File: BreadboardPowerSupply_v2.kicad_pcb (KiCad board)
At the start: 2 copper layers, 30.1 x 52.2 mm, 15 parts, among them J1 Barrel_Jack_Switch, J2 Conn_02x02_Odd_Even, J3 Conn_02x02_Odd_Even, SW1 SW_DPDT_x2, U1 LM7805_TO220

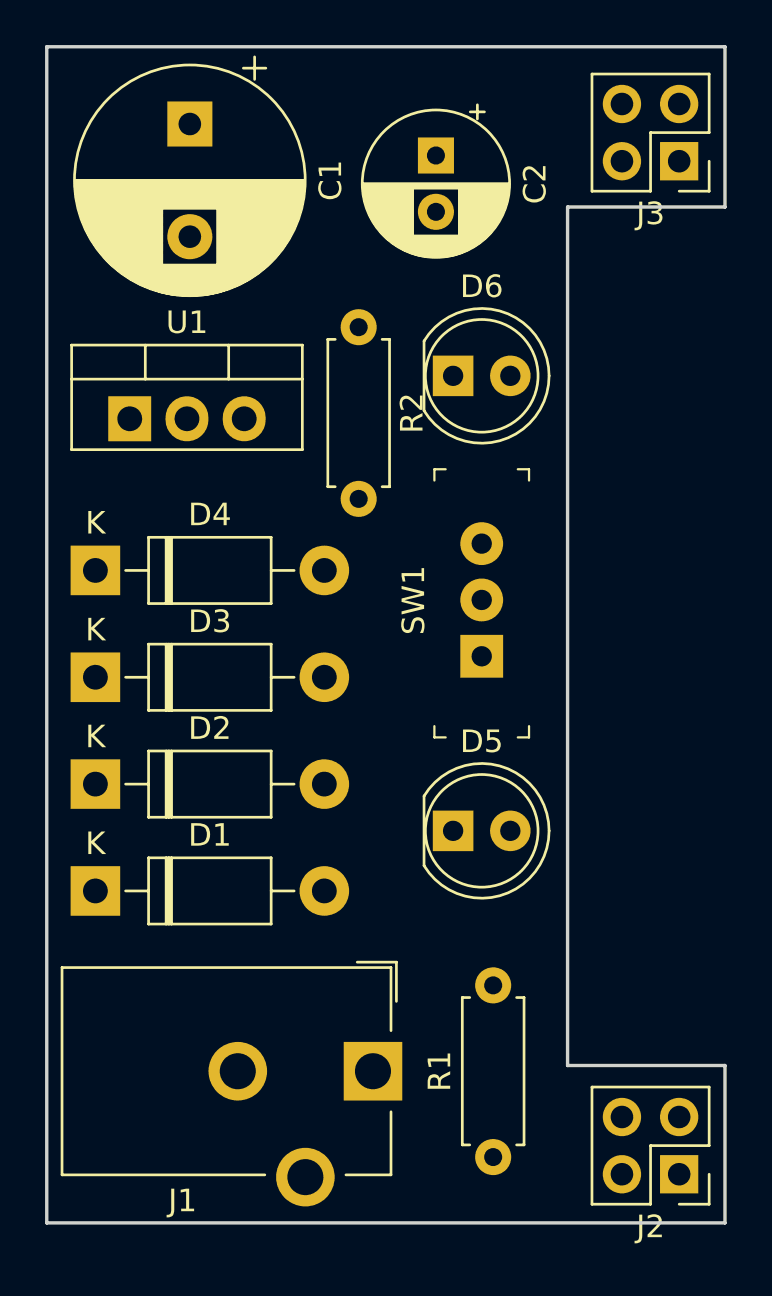
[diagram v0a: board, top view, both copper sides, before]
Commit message: Tracing is complete.
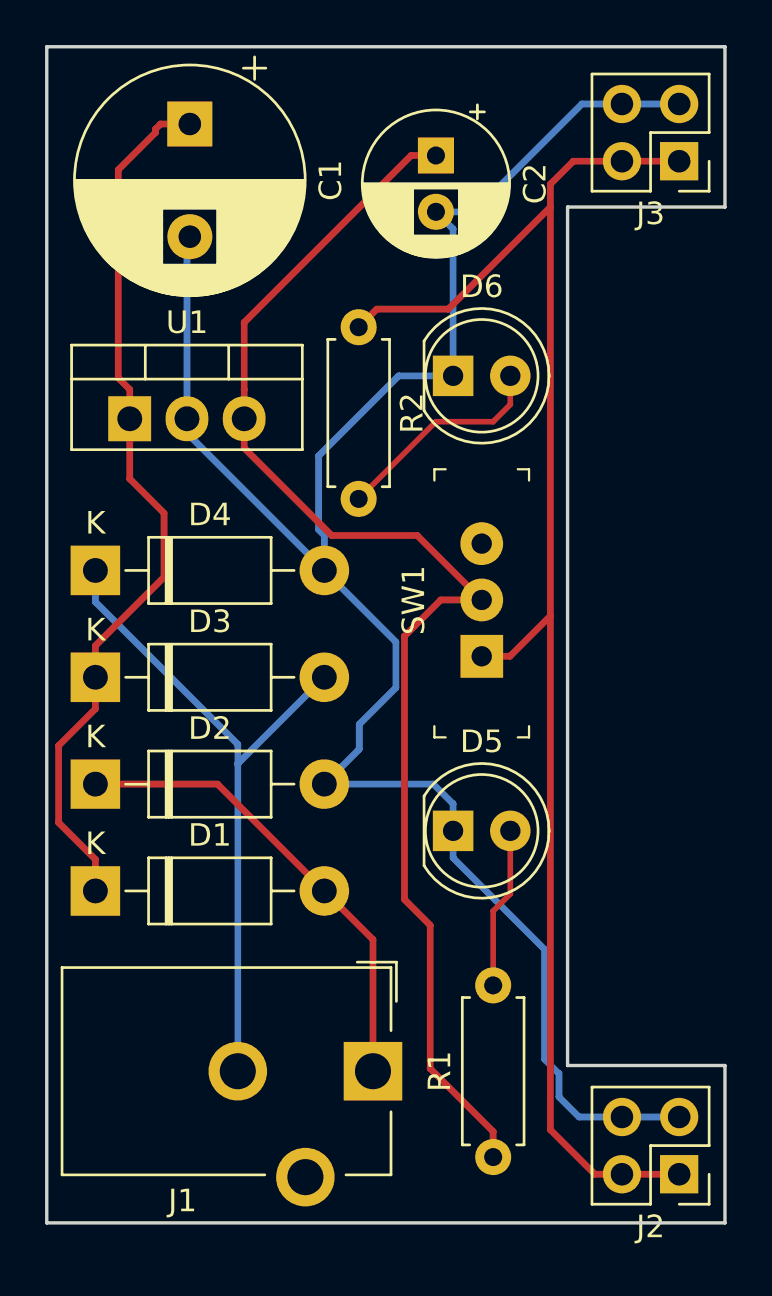
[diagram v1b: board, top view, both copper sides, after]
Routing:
- net /V-: track 0.00 -> 89.2 mm
- net /Vout2: track 0.00 -> 69.1 mm
- net /Vout1: track 0.00 -> 59.3 mm
- net /Vin: track 0.00 -> 39.6 mm
- net /V2: track 0.00 -> 30.3 mm
- net /V1: track 0.00 -> 21.0 mm
- net Net-(D6-Pad2): track 0.00 -> 9.74 mm
- net Net-(D5-Pad2): track 0.00 -> 7.17 mm
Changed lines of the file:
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@@
     (thickness 1.6)
     (drawings 13)
-    (tracks 0)
+    (tracks 93)
     (zones 0)
     (modules 15)
@@
     (uvia_dia 0.3)
     (uvia_drill 0.1)
-    (add_net /V-)
-    (add_net /V1)
-    (add_net /V2)
-    (add_net /Vin)
-    (add_net /Vout1)
-    (add_net /Vout2)
     (add_net "Net-(D5-Pad2)")
     (add_net "Net-(D6-Pad2)")
@@
     (uvia_dia 0.3)
     (uvia_drill 0.1)
+    (add_net /V-)
+    (add_net /V1)
+    (add_net /V2)
+    (add_net /Vin)
+    (add_net /Vout1)
+    (add_net /Vout2)
   )
   (module Capacitor_THT:CP_Radial_D6.3mm_P2.50mm (layer F.Cu)
@@
   (gr_line (start 36.957 159.385) (end 67.056 159.385) (layer Edge.Cuts) (width 0.15))
   (gr_line (start 36.957 107.188) (end 36.957 159.385) (layer Edge.Cuts) (width 0.15))
+  (segment (start 37.48201 141.61901) (end 39.116 143.253) (width 0.3) (layer F.Cu) (net 1))
+  (segment (start 37.48201 138.204323) (end 37.48201 141.61901) (width 0.3) (layer F.Cu) (net 1))
+  (segment (start 39.116 136.570333) (end 37.48201 138.204323) (width 0.3) (layer F.Cu) (net 1))
+  (segment (start 39.116 143.253) (end 39.116 144.653) (width 0.3) (layer F.Cu) (net 1))
+  (segment (start 39.116 135.170333) (end 39.116 136.570333) (width 0.3) (layer F.Cu) (net 1))
+  (segment (start 39.116 133.770333) (end 42.164 130.722333) (width 0.3) (layer F.Cu) (net 1))
+  (segment (start 39.116 135.170333) (end 39.116 133.770333) (width 0.3) (layer F.Cu) (net 1))
+  (segment (start 42.164 130.722333) (end 42.164 127.889) (width 0.3) (layer F.Cu) (net 1))
+  (segment (start 40.64 126.365) (end 40.64 123.698) (width 0.3) (layer F.Cu) (net 1))
+  (segment (start 42.164 127.889) (end 40.64 126.365) (width 0.3) (layer F.Cu) (net 1))
+  (segment (start 42.007 110.617) (end 43.307 110.617) (width 0.3) (layer F.Cu) (net 1))
+  (segment (start 40.132 112.649) (end 41.783 110.998) (width 0.3) (layer F.Cu) (net 1))
+  (segment (start 40.64 122.398) (end 40.132 121.89) (width 0.3) (layer F.Cu) (net 1))
+  (segment (start 40.64 123.698) (end 40.64 122.398) (width 0.3) (layer F.Cu) (net 1))
+  (segment (start 40.132 121.89) (end 40.132 112.649) (width 0.3) (layer F.Cu) (net 1))
+  (segment (start 41.783 110.841) (end 42.007 110.617) (width 0.3) (layer F.Cu) (net 1))
+  (segment (start 41.783 110.998) (end 41.783 110.841) (width 0.3) (layer F.Cu) (net 1))
+  (segment (start 43.18 124.333) (end 43.18 123.698) (width 0.3) (layer B.Cu) (net 2))
+  (segment (start 49.276 130.429) (end 43.18 124.333) (width 0.3) (layer B.Cu) (net 2))
+  (segment (start 54.991 140.786) (end 54.991 141.986) (width 0.3) (layer B.Cu) (net 2))
+  (segment (start 54.116666 139.911666) (end 54.991 140.786) (width 0.3) (layer B.Cu) (net 2))
+  (segment (start 49.276 139.911666) (end 54.116666 139.911666) (width 0.3) (layer B.Cu) (net 2))
+  (segment (start 54.991 143.186) (end 59.055 147.25) (width 0.3) (layer B.Cu) (net 2))
+  (segment (start 54.991 141.986) (end 54.991 143.186) (width 0.3) (layer B.Cu) (net 2))
+  (segment (start 59.055 152.126476) (end 59.69 152.761476) (width 0.3) (layer B.Cu) (net 2))
+  (segment (start 59.055 147.25) (end 59.055 152.126476) (width 0.3) (layer B.Cu) (net 2))
+  (segment (start 59.69 152.761476) (end 59.69 153.797) (width 0.3) (layer B.Cu) (net 2))
+  (segment (start 60.579 154.686) (end 62.484 154.686) (width 0.3) (layer B.Cu) (net 2))
+  (segment (start 59.69 153.797) (end 60.579 154.686) (width 0.3) (layer B.Cu) (net 2))
+  (segment (start 62.484 154.686) (end 65.024 154.686) (width 0.3) (layer B.Cu) (net 2))
+  (segment (start 50.826001 138.361665) (end 50.826001 137.260999) (width 0.3) (layer B.Cu) (net 2))
+  (segment (start 49.276 139.911666) (end 50.826001 138.361665) (width 0.3) (layer B.Cu) (net 2))
+  (segment (start 50.826001 137.260999) (end 52.451 135.636) (width 0.3) (layer B.Cu) (net 2))
+  (segment (start 52.451 133.604) (end 49.276 130.429) (width 0.3) (layer B.Cu) (net 2))
+  (segment (start 52.451 135.636) (end 52.451 133.604) (width 0.3) (layer B.Cu) (net 2))
+  (segment (start 49.276 128.873366) (end 49.022 128.619366) (width 0.3) (layer B.Cu) (net 2))
+  (segment (start 49.276 130.429) (end 49.276 128.873366) (width 0.3) (layer B.Cu) (net 2))
+  (segment (start 49.022 128.619366) (end 49.022 125.349) (width 0.3) (layer B.Cu) (net 2))
+  (segment (start 52.578 121.793) (end 54.991 121.793) (width 0.3) (layer B.Cu) (net 2))
+  (segment (start 49.022 125.349) (end 52.578 121.793) (width 0.3) (layer B.Cu) (net 2))
+  (segment (start 54.991 115.276) (end 54.229 114.514) (width 0.3) (layer B.Cu) (net 2))
+  (segment (start 54.991 121.793) (end 54.991 115.276) (width 0.3) (layer B.Cu) (net 2))
+  (segment (start 43.18 115.744) (end 43.307 115.617) (width 0.3) (layer B.Cu) (net 2))
+  (segment (start 43.18 123.698) (end 43.18 115.744) (width 0.3) (layer B.Cu) (net 2))
+  (segment (start 54.229 114.514) (end 55.92 114.514) (width 0.3) (layer B.Cu) (net 2))
+  (segment (start 55.92 114.514) (end 60.706 109.728) (width 0.3) (layer B.Cu) (net 2))
+  (segment (start 60.706 109.728) (end 62.484 109.728) (width 0.3) (layer B.Cu) (net 2))
+  (segment (start 62.484 109.728) (end 65.024 109.728) (width 0.3) (layer B.Cu) (net 2))
+  (segment (start 56.769 148.844) (end 56.769 145.542) (width 0.25) (layer F.Cu) (net 3))
+  (segment (start 57.531 144.78) (end 57.531 141.986) (width 0.25) (layer F.Cu) (net 3))
+  (segment (start 56.769 145.542) (end 57.531 144.78) (width 0.25) (layer F.Cu) (net 3))
+  (segment (start 57.531 123.065792) (end 56.769 123.827792) (width 0.25) (layer F.Cu) (net 4))
+  (segment (start 57.531 121.793) (end 57.531 123.065792) (width 0.25) (layer F.Cu) (net 4))
+  (segment (start 54.226208 123.827792) (end 50.8 127.254) (width 0.25) (layer F.Cu) (net 4))
+  (segment (start 56.769 123.827792) (end 54.226208 123.827792) (width 0.25) (layer F.Cu) (net 4))
+  (segment (start 51.435 146.812) (end 49.276 144.653) (width 0.3) (layer F.Cu) (net 7))
+  (segment (start 51.435 152.654) (end 51.435 146.812) (width 0.3) (layer F.Cu) (net 7))
+  (segment (start 44.534666 139.911666) (end 39.116 139.911666) (width 0.3) (layer F.Cu) (net 7))
+  (segment (start 49.276 144.653) (end 44.534666 139.911666) (width 0.3) (layer F.Cu) (net 7))
+  (segment (start 45.435 139.011333) (end 49.276 135.170333) (width 0.3) (layer B.Cu) (net 8))
+  (segment (start 45.435 152.654) (end 45.435 139.011333) (width 0.3) (layer B.Cu) (net 8))
+  (segment (start 45.435 138.148) (end 45.435 139.011333) (width 0.3) (layer B.Cu) (net 8))
+  (segment (start 39.116 131.829) (end 45.435 138.148) (width 0.3) (layer B.Cu) (net 8))
+  (segment (start 39.116 130.429) (end 39.116 131.829) (width 0.3) (layer B.Cu) (net 8))
+  (segment (start 51.599999 118.834001) (end 54.774999 118.834001) (width 0.3) (layer F.Cu) (net 9))
+  (segment (start 50.8 119.634) (end 51.599999 118.834001) (width 0.3) (layer F.Cu) (net 9))
+  (segment (start 54.774999 118.834001) (end 59.309 114.3) (width 0.3) (layer F.Cu) (net 9))
+  (segment (start 59.309 114.3) (end 59.309 113.284) (width 0.3) (layer F.Cu) (net 9))
+  (segment (start 60.325 112.268) (end 62.484 112.268) (width 0.3) (layer F.Cu) (net 9))
+  (segment (start 59.309 113.284) (end 60.325 112.268) (width 0.3) (layer F.Cu) (net 9))
+  (segment (start 62.484 112.268) (end 65.024 112.268) (width 0.3) (layer F.Cu) (net 9))
+  (segment (start 59.309 132.441) (end 59.309 114.3) (width 0.3) (layer F.Cu) (net 9))
+  (segment (start 57.511 134.239) (end 59.309 132.441) (width 0.3) (layer F.Cu) (net 9))
+  (segment (start 56.261 134.239) (end 57.511 134.239) (width 0.3) (layer F.Cu) (net 9))
+  (segment (start 59.309 155.253081) (end 59.309 132.441) (width 0.3) (layer F.Cu) (net 9))
+  (segment (start 61.281919 157.226) (end 59.309 155.253081) (width 0.3) (layer F.Cu) (net 9))
+  (segment (start 62.484 157.226) (end 61.281919 157.226) (width 0.3) (layer F.Cu) (net 9))
+  (segment (start 65.024 157.226) (end 62.484 157.226) (width 0.3) (layer F.Cu) (net 9))
+  (segment (start 45.72 122.398) (end 45.72 123.698) (width 0.3) (layer F.Cu) (net 10))
+  (segment (start 45.72 119.423) (end 45.72 122.398) (width 0.3) (layer F.Cu) (net 10))
+  (segment (start 53.129 112.014) (end 45.72 119.423) (width 0.3) (layer F.Cu) (net 10))
+  (segment (start 54.229 112.014) (end 53.129 112.014) (width 0.3) (layer F.Cu) (net 10))
+  (segment (start 45.72 124.998) (end 45.72 123.698) (width 0.3) (layer F.Cu) (net 10))
+  (segment (start 49.600999 128.878999) (end 45.72 124.998) (width 0.3) (layer F.Cu) (net 10))
+  (segment (start 53.400999 128.878999) (end 49.600999 128.878999) (width 0.3) (layer F.Cu) (net 10))
+  (segment (start 56.261 131.739) (end 53.400999 128.878999) (width 0.3) (layer F.Cu) (net 10))
+  (segment (start 56.769 155.33263) (end 53.975 152.53863) (width 0.3) (layer F.Cu) (net 10))
+  (segment (start 56.769 156.464) (end 56.769 155.33263) (width 0.3) (layer F.Cu) (net 10))
+  (segment (start 53.975 152.53863) (end 53.975 146.177) (width 0.3) (layer F.Cu) (net 10))
+  (segment (start 53.975 146.177) (end 52.832 145.034) (width 0.3) (layer F.Cu) (net 10))
+  (segment (start 52.832 145.034) (end 52.832 133.35) (width 0.3) (layer F.Cu) (net 10))
+  (segment (start 54.443 131.739) (end 56.261 131.739) (width 0.3) (layer F.Cu) (net 10))
+  (segment (start 52.832 133.35) (end 54.443 131.739) (width 0.3) (layer F.Cu) (net 10))
 )
